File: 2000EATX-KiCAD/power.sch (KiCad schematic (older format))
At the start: 44 parts, among them CN400 ATX-24, J9000 POWER_SWITCH, U9000 MC7905, U9001 74HC14, U9002 74HC74

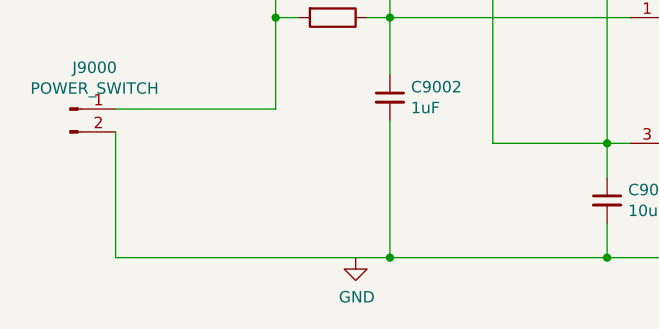
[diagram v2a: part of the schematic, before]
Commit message: Add files via upload
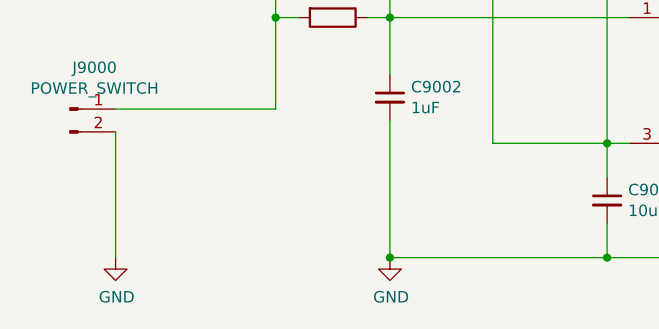
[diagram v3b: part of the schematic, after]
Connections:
- net GND: now also C9002.2, C9003.2, J9000.2 (Pin_2), U9001.7 (GND), U9002.7 (GND)
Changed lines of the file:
@@
 L power:GND #PWR0169
 U 1 1 60A6AF77
-P 2150 6800
-F 0 "#PWR0169" H 2150 6550 50  0001 C CNN
-F 1 "GND" H 2155 6627 50  0000 C CNN
-F 2 "" H 2150 6800 50  0001 C CNN
-F 3 "" H 2150 6800 50  0001 C CNN
-	1    2150 6800
+P 2300 6800
+F 0 "#PWR0169" H 2300 6550 50  0001 C CNN
+F 1 "GND" H 2305 6627 50  0000 C CNN
+F 2 "" H 2300 6800 50  0001 C CNN
+F 3 "" H 2300 6800 50  0001 C CNN
+	1    2300 6800
 	1    0    0    -1
 $EndComp
@@
 Wire Wire Line
 	2100 1850 2250 1850
-Wire Wire Line
-	1100 6800 2300 6800
 $Comp
 L Mechanical:MountingHole_Pad H1
@@
 Text Notes 9050 3250 0    118  ~ 0
 MOUNTING\nHOLES
+$Comp
+L power:GND #PWR0177
+U 1 1 608A0106
+P 1100 6800
+F 0 "#PWR0177" H 1100 6550 50  0001 C CNN
+F 1 "GND" H 1105 6627 50  0000 C CNN
+F 2 "" H 1100 6800 50  0001 C CNN
+F 3 "" H 1100 6800 50  0001 C CNN
+	1    1100 6800
+	1    0    0    -1
+$EndComp
 $EndSCHEMATC
